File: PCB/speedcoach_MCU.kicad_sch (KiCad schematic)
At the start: 24 parts, among them J3 Conn_01x04_Male, J4 USB_B_Micro, J5 440055-2, SW1 1825027-8, SW2 1825027-8, SW3 1825027-8, U8 MCP73831, U9 STM32L051x6

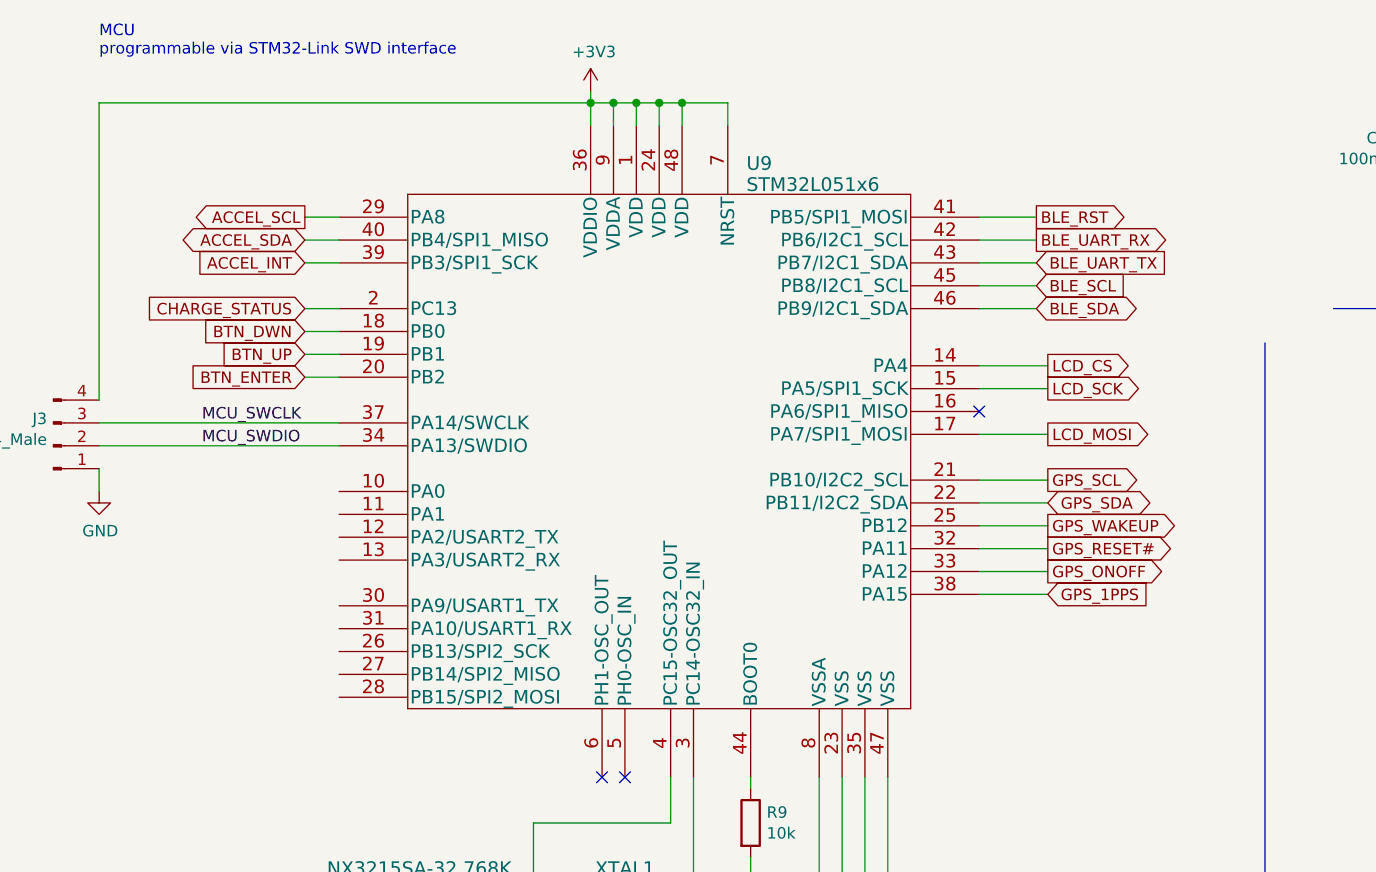
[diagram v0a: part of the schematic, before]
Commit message: revised MCU
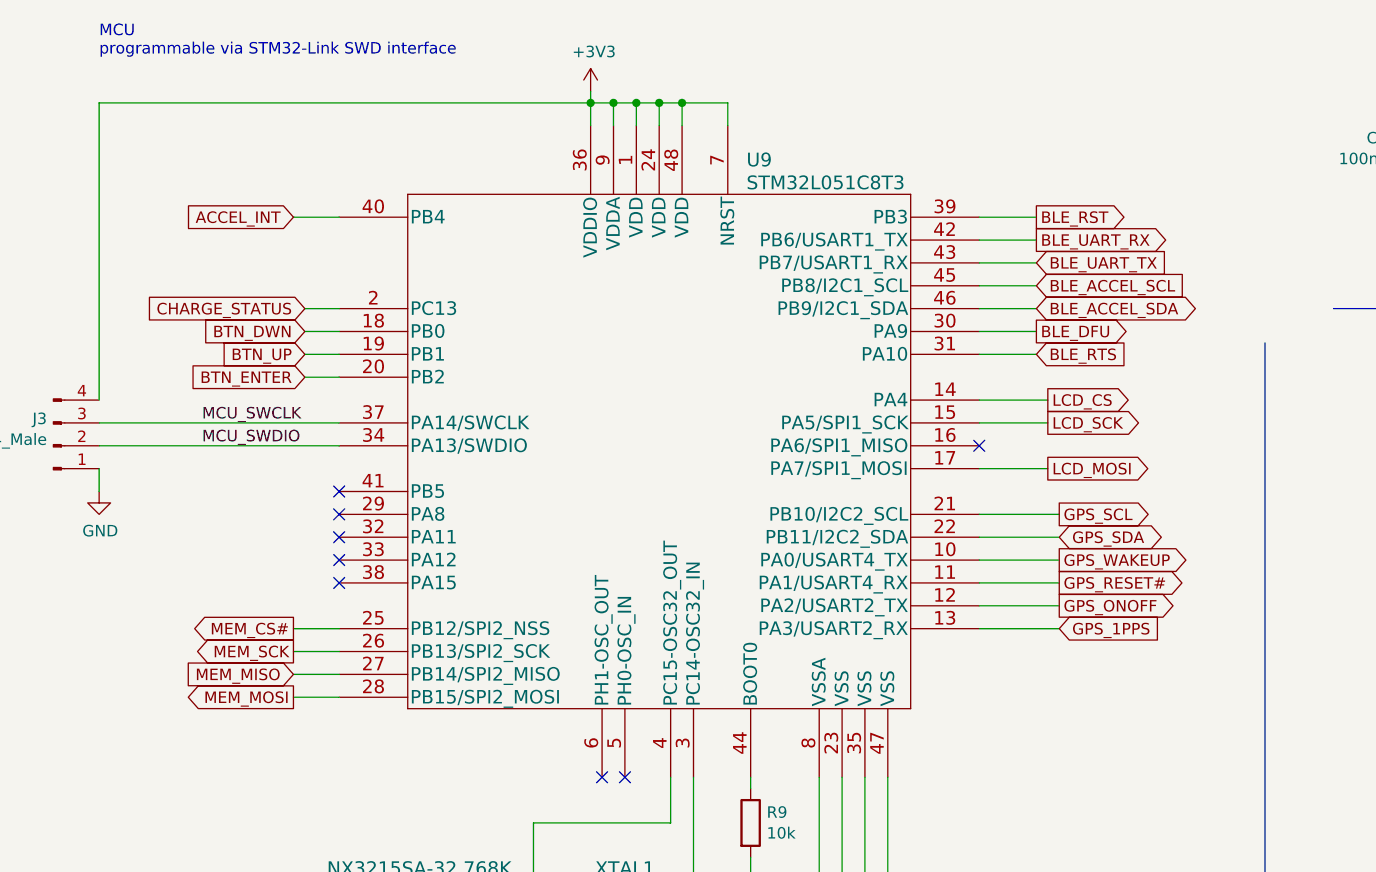
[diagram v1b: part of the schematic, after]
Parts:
- removed U9: STM32L051x6, speedcoach:STM32L071C8T6, symbol speedcoach:STM32L051x6
- added U9: STM32L051C8T3, symbol speedcoach:STM32L051C8T3
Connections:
- net +3V3: now also U9.1 (VDD), U9.24 (VDD), U9.36 (VDDIO), U9.48 (VDD), U9.7 (NRST), U9.9 (VDDA)
- net ACCEL_INT: now also U9.40 (PB4)
- net BLE_RST: now also U9.39 (PB3)
- net BLE_UART_RX: now also U9.42 (PB6/USART1_TX)
- net BLE_UART_TX: now also U9.43 (PB7/USART1_RX)
- net BTN_DWN: now also U9.18 (PB0)
- net BTN_ENTER: now also U9.20 (PB2)
- net BTN_UP: now also U9.19 (PB1)
- net CHARGE_STATUS: now also U9.2 (PC13)
- net GND: now also U9.23 (VSS), U9.35 (VSS), U9.47 (VSS), U9.8 (VSSA)
- net GPS_1PPS: now also U9.13 (PA3/USART2_RX)
- net GPS_ONOFF: now also U9.12 (PA2/USART2_TX)
- net GPS_RESET#: now also U9.11 (PA1/USART4_RX)
- net GPS_SCL: now also U9.21 (PB10/I2C2_SCL)
- net GPS_SDA: now also U9.22 (PB11/I2C2_SDA)
- net GPS_WAKEUP: now also U9.10 (PA0/USART4_TX)
- net LCD_CS: now also U9.14 (PA4)
- net LCD_MOSI: now also U9.17 (PA7/SPI1_MOSI)
- net LCD_SCK: now also U9.15 (PA5/SPI1_SCK)
- net MCU_SWCLK: now also U9.37 (PA14/SWCLK)
- net MCU_SWDIO: now also U9.34 (PA13/SWDIO)
- net at R9.1: now also U9.44 (BOOT0)
- net at C2.2, XTAL1.1: now also U9.4 (PC15-OSC32_OUT)
- net at C3.2, XTAL1.2: now also U9.3 (PC14-OSC32_IN)
- new net BLE_ACCEL_SCL: U9.45 (PB8/I2C1_SCL)
- new net BLE_ACCEL_SDA: U9.46 (PB9/I2C1_SDA)
- new net BLE_DFU: U9.30 (PA9)
- new net BLE_RTS: U9.31 (PA10)
- new net MEM_CS#: U9.25 (PB12/SPI2_NSS)
- new net MEM_MISO: U9.27 (PB14/SPI2_MISO)
- new net MEM_MOSI: U9.28 (PB15/SPI2_MOSI)
- new net MEM_SCK: U9.26 (PB13/SPI2_SCK)
- no-connect marks 6 -> 11
